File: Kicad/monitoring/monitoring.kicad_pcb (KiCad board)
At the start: 2 copper layers, 51.1 x 98.7 mm, 21 parts, among them J1 Module1, J2 Module2, J3 Module3, J4 buttons, J5 Display, J6 Display, J7 DC_in_outout, U1 4052, U3 L7805, U4 L7805

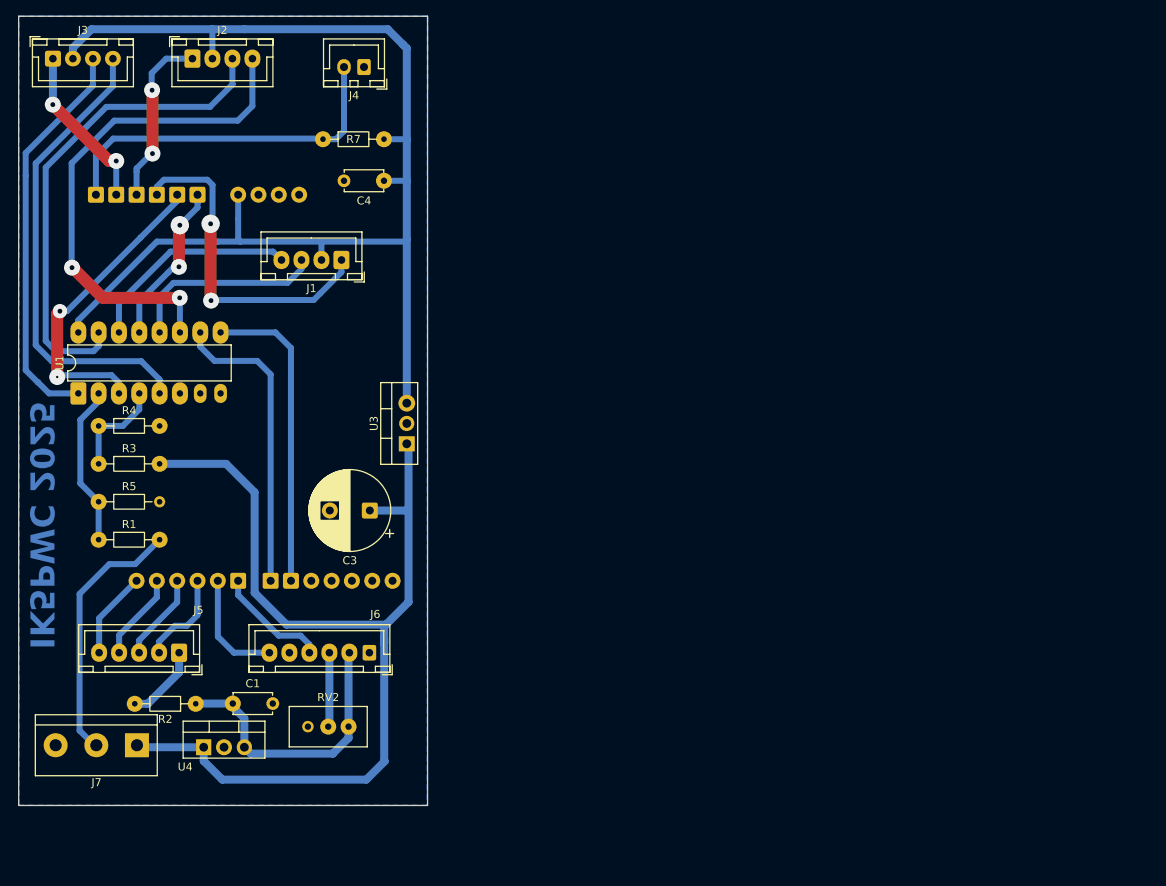
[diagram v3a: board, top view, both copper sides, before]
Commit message: Update UPSMonitor.ino, datatypes.h, io.cpp, and 18 more files
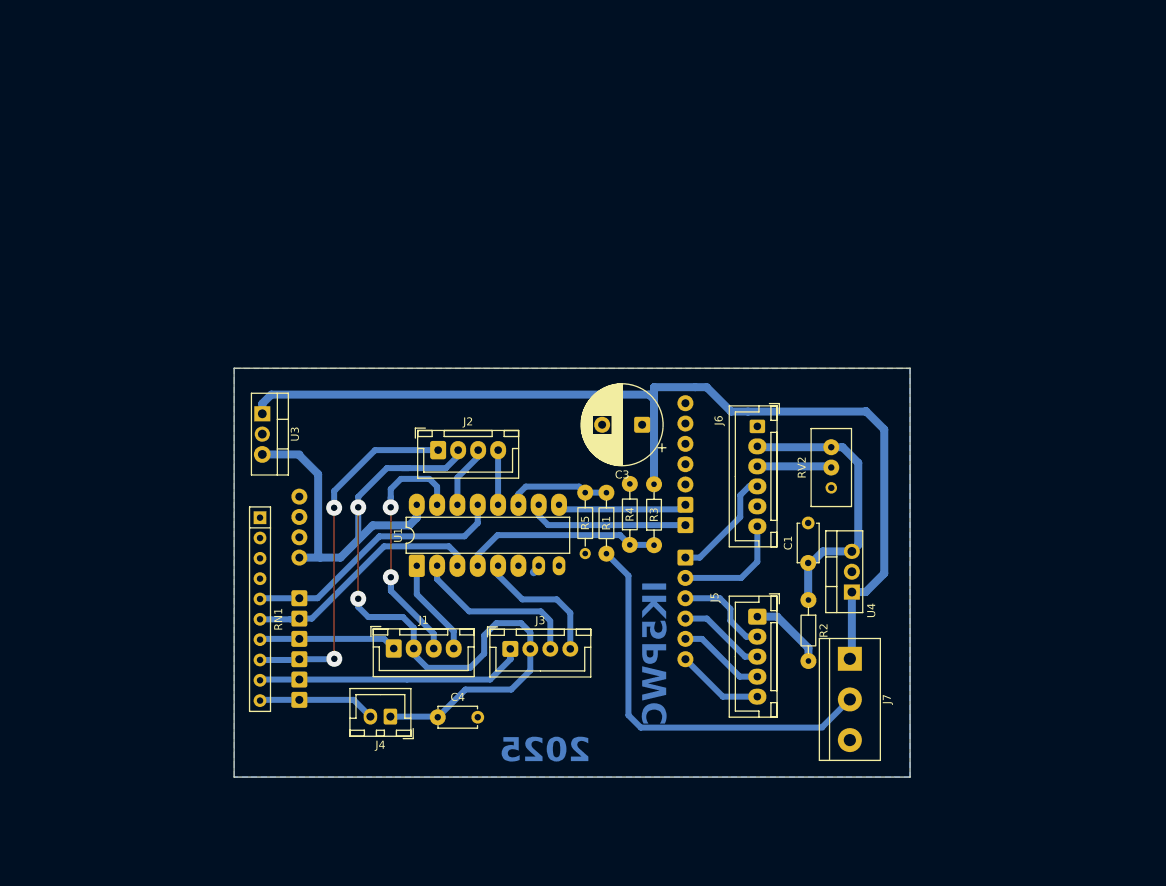
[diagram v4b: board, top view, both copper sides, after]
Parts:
- removed R7: 10K, Resistor_THT:R_Axial_DIN0204_L3.6mm_D1.6mm_P7.62mm_Horizontal
- added RN1: 4K7, Resistor_THT:R_Array_SIP10, F.Cu at (47.9, 80.0)
- R1, R3: value 3K3 -> 3K
- moved J3 93.3 mm to (79.2, 96.4)
- moved J7 89.8 mm to (121.7, 97.7), turned to -90 degrees
- moved U4 83.3 mm to (121.9, 89.3), turned to 90 degrees
- moved J4 81.3 mm to (64.2, 104.9)
- moved R2 77.7 mm to (116.5, 90.3), turned to -90 degrees
- moved C1 74.0 mm to (116.4, 85.7), turned to 90 degrees
- moved J5 72.4 mm to (110.1, 92.4), turned to -90 degrees
- moved R3 70.2 mm to (97.2, 83.5), turned to 90 degrees
- moved RV2 69.7 mm to (119.3, 71.2), turned to 90 degrees
- moved R4 68.0 mm to (94.2, 83.4), turned to 90 degrees
- moved C4 67.4 mm to (70.1, 105.0), turned to 0 degrees
- moved R1 63.7 mm to (91.2, 76.9), turned to -90 degrees
- moved R5 60.8 mm to (88.6, 76.9), turned to -90 degrees
- moved J2 57.8 mm to (70.2, 71.6)
- moved J6 56.1 mm to (110.1, 68.6), turned to -90 degrees
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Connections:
- net /dc_Vout renamed /ups_Vout
- net /ps_out renamed Net-(J7-Pin_2)
- J4 pad 1: GND -> +5VA
- R1 pad 1: /ps_Vin -> /ps_Vout
- R5 pad 1: /ps_Vin -> /ps_Vout
- U1 pad 1: /m3_Iout -> /m1_Ibat
- U1 pad 11: /m2_Ibat -> /ps_Vout
- U1 pad 12: /m1_Iout -> /m2_Ibat
- U1 pad 14: /m1_Ibat -> /m2_Iout
- U1 pad 15: /m2_Iout -> /m1_Iout
- U1 pad 2: /ps_Vin -> /m3_Iout
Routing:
- net /m2_Ibat: track 64.6 -> 6.84 mm, vias 2 -> 0
- net /m2_Iout: track 61.9 -> 8.00 mm
- net /m3_Ibat: track 58.8 -> 16.7 mm
- net /PUSH: track 45.1 -> 14.7 mm
- net /m3_Iout: track 50.2 -> 21.3 mm
- net /m1_Vbat: track 43.1 -> 17.2 mm, vias 2 -> 0
- net /m2_Vbat: track 22.0 -> 44.9 mm
- net /BCD-2: track 38.7 -> 16.3 mm
- net /ps_Vin: track 20.2 -> 0.00 mm
- net Net-(J7-Pin_2): track 33.2 -> 51.1 mm
- net /BCD-1: track 37.8 -> 20.6 mm
- net +5VA: track 154.0 -> 137.9 mm, vias 0 -> 2
- net /m1_Ibat: track 27.1 -> 12.3 mm
- net /ps_Vout: track 0.00 -> 13.1 mm
- net /m3_Vbat: track 20.8 -> 33.7 mm, vias 2 -> 0
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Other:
- board size 51.1 x 98.7 mm -> 84.5 x 51.1 mm
- board text added: "2025"
- board text added: "IK5PWC"
- board text removed: "IK5PWC 2025"

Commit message: Update .sproject, io.cpp, io.h, and 29 more files
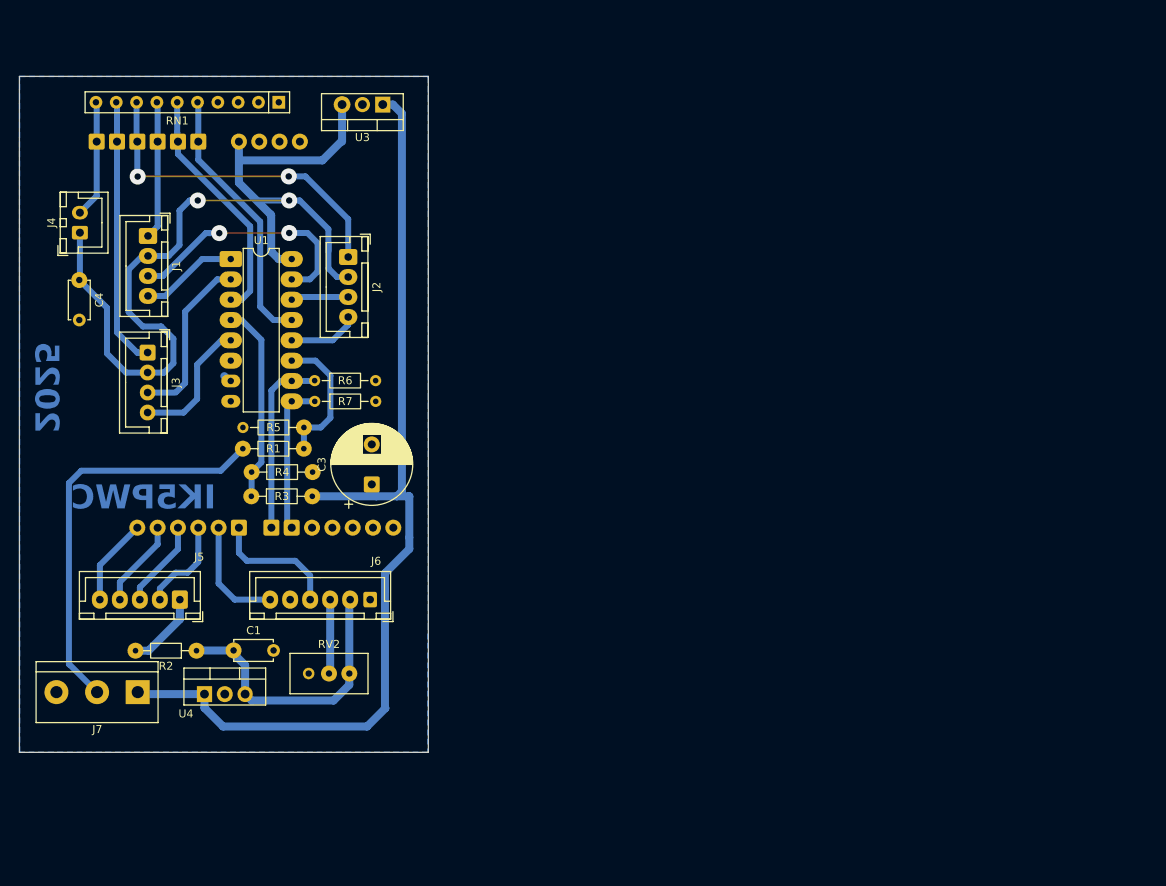
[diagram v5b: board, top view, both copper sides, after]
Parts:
- added R6: 100K, Resistor_THT:R_Axial_DIN0204_L3.6mm_D1.6mm_P7.62mm_Horizontal, F.Cu at (54.8, 62.9)
- added R7: 100K, Resistor_THT:R_Axial_DIN0204_L3.6mm_D1.6mm_P7.62mm_Horizontal, F.Cu at (54.8, 65.5)
- moved J7 89.1 mm to (32.6, 101.8), turned to 180 degrees
- moved U4 81.9 mm to (41.0, 102.1), turned to 0 degrees
- moved R2 76.8 mm to (40.0, 96.7), turned to 180 degrees
- moved C1 72.7 mm to (44.6, 96.6), turned to 0 degrees
- moved J5 72.2 mm to (37.9, 90.3), turned to 180 degrees
- moved J4 71.9 mm to (25.4, 44.4), turned to 90 degrees
- moved C4 70.7 mm to (25.3, 50.3), turned to -90 degrees
- moved RV2 66.6 mm to (59.1, 99.5), turned to 0 degrees
- moved J1 60.0 mm to (33.9, 44.8), turned to -90 degrees
- moved J3 58.5 mm to (33.9, 59.4), turned to -90 degrees
- moved J6 53.0 mm to (61.7, 90.3), turned to 180 degrees
- moved RN1 52.0 mm to (50.3, 28.1), turned to 180 degrees
- moved R3 50.7 mm to (46.8, 77.4), turned to 0 degrees
- moved R4 48.1 mm to (46.9, 74.3), turned to 0 degrees
- moved U1 44.8 mm to (44.3, 47.7), turned to 0 degrees
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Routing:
- net /ps_Vout: track 13.1 -> 17.4 mm
- net /BCD-1: track 20.6 -> 23.5 mm
- net /BCD-2: track 16.3 -> 19.2 mm
- net /m2_Vbat: track 44.9 -> 42.1 mm
- net +5VA: track 137.9 -> 135.5 mm
- net /m2_Ibat: track 6.84 -> 8.84 mm
- net /LCD_RS: track 14.3 -> 16.2 mm
- net /m2_Iout: track 8.00 -> 7.29 mm
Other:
- board size 84.5 x 51.1 mm -> 51.1 x 84.5 mm
